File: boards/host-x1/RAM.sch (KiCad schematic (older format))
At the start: 0 parts

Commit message: Continued work on power supply
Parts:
- added U2: XC7A100T-1FTG256C, symbol XC7AxT-xFTG256x
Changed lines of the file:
@@
 $Descr A4 11693 8268
 encoding utf-8
-Sheet 1 4
+Sheet 3 5
 Title "STARSHIPRAIDER Single-Lane Host"
 Date "2017-05-04"
@@
 Comment4 ""
 $EndDescr
+$Comp
+L XC7AxT-xFTG256x U2
+U 6 1 590BFFBD
+P 1750 6050
+F 0 "U2" H 3128 8558 60  0000 L CNN
+F 1 "XC7A100T-1FTG256C" H 3128 8452 60  0000 L CNN
+F 2 "" H 1750 6050 60  0000 C CNN
+F 3 "" H 1750 6050 60  0000 C CNN
+	6    1750 6050
+	1    0    0    -1
+$EndComp
+$Comp
+L XC7AxT-xFTG256x U2
+U 5 1 590C013F
+P 4850 6000
+F 0 "U2" H 6228 8508 60  0000 L CNN
+F 1 "XC7A100T-1FTG256C" H 6228 8402 60  0000 L CNN
+F 2 "" H 4850 6000 60  0000 C CNN
+F 3 "" H 4850 6000 60  0000 C CNN
+	5    4850 6000
+	1    0    0    -1
+$EndComp
 $EndSCHEMATC

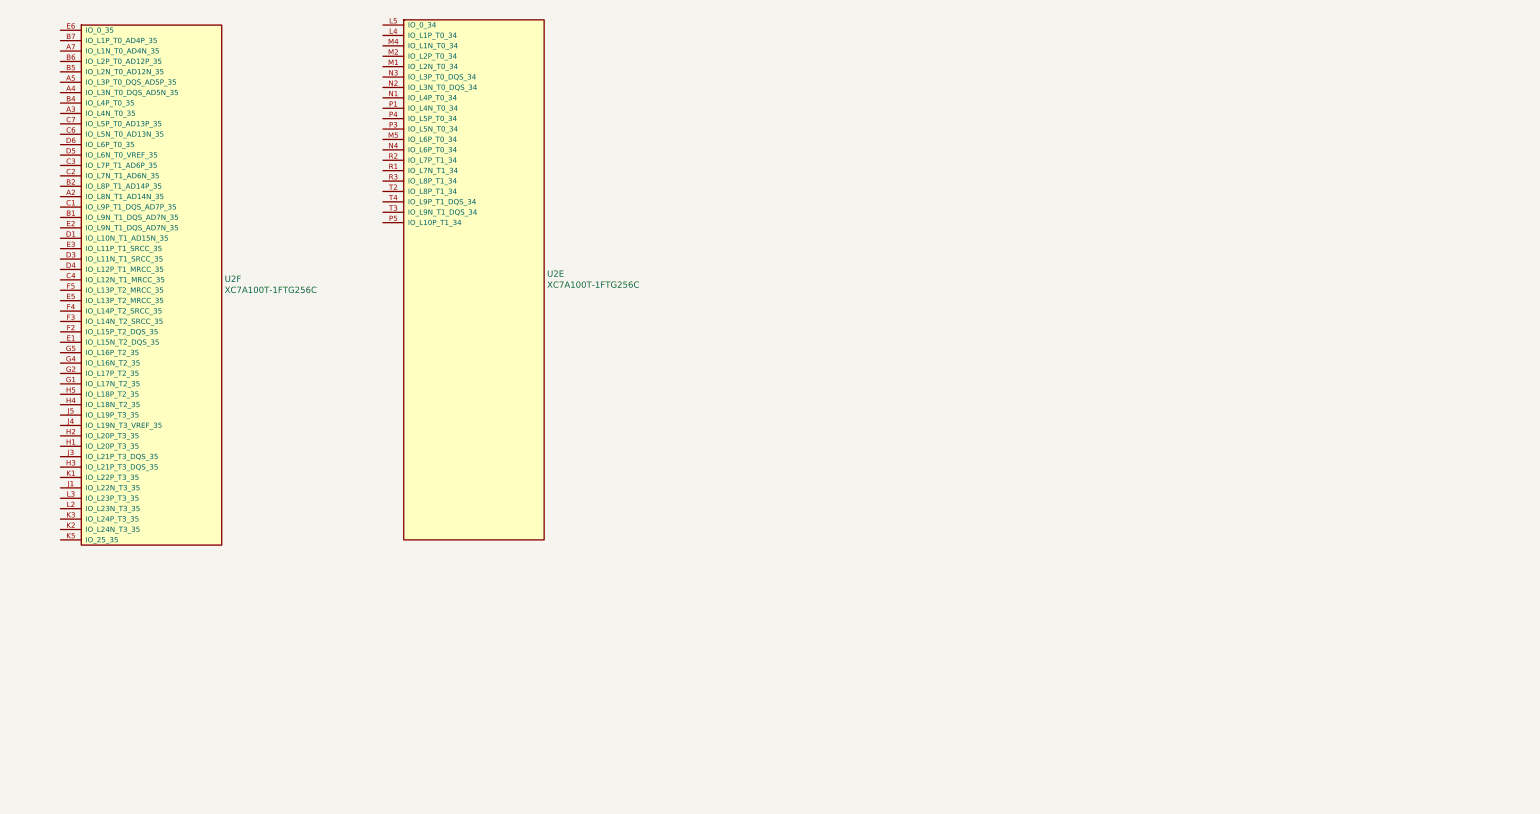
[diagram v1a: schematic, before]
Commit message: Initial work on RAM
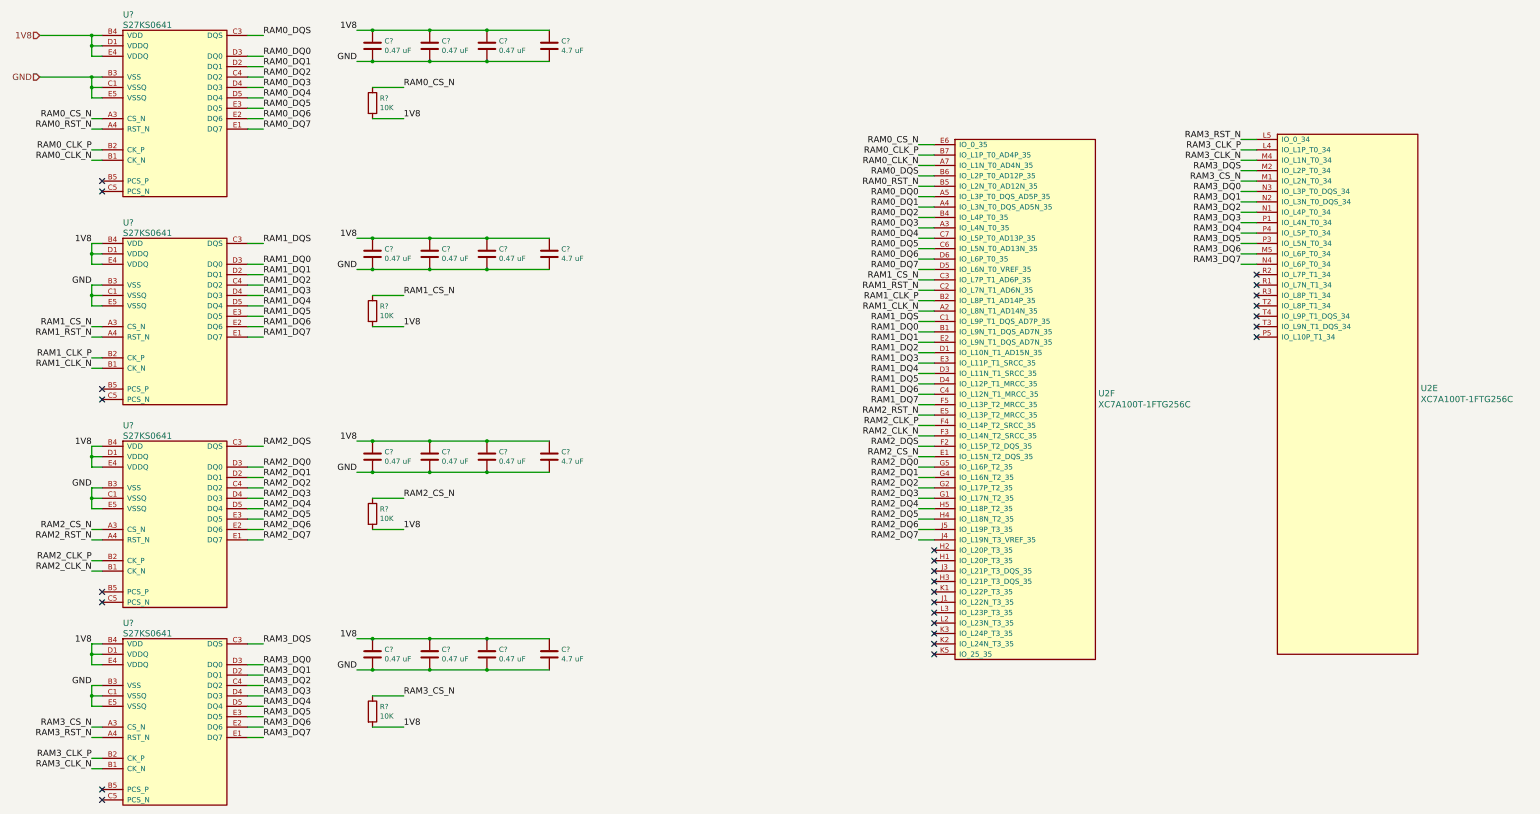
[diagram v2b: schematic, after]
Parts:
- added C? (x12): 0.47 uF, symbol C
- added C? (x4): 4.7 uF, symbol C
- added R? (x4): 10K, symbol R
- added U? (x4): S27KS0641, symbol S27KS0641
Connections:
- net RAM1_CLK_N: now reaches U2.A2 (IO_L8N_T1_AD14N_35)
- net RAM1_CLK_N: now also U?.B1 (CK_N)
- net RAM0_DQ3: now reaches U2.A3 (IO_L4N_T0_35)
- net RAM0_DQ3: now also U?.D4 (DQ3)
- net RAM0_DQ1: now reaches U2.A4 (IO_L3N_T0_DQS_AD5N_35)
- net RAM0_DQ1: now also U?.D2 (DQ1)
- net RAM0_DQ0: now reaches U2.A5 (IO_L3P_T0_DQS_AD5P_35)
- net RAM0_DQ0: now also U?.D3 (DQ0)
- net RAM0_CLK_N: now reaches U2.A7 (IO_L1N_T0_AD4N_35)
- net RAM0_CLK_N: now also U?.B1 (CK_N)
- net RAM1_DQ0: now reaches U2.B1 (IO_L9N_T1_DQS_AD7N_35)
- net RAM1_DQ0: now also U?.D3 (DQ0)
- net RAM1_CLK_P: now reaches U2.B2 (IO_L8P_T1_AD14P_35)
- net RAM1_CLK_P: now also U?.B2 (CK_P)
- net RAM0_DQ2: now reaches U2.B4 (IO_L4P_T0_35)
- net RAM0_DQ2: now also U?.C4 (DQ2)
- net RAM0_RST_N: now reaches U2.B5 (IO_L2N_T0_AD12N_35)
- net RAM0_RST_N: now also U?.A4 (RST_N)
- net RAM0_DQS: now reaches U2.B6 (IO_L2P_T0_AD12P_35)
- net RAM0_DQS: now also U?.C3 (DQS)
- net RAM0_CLK_P: now reaches U2.B7 (IO_L1P_T0_AD4P_35)
- net RAM0_CLK_P: now also U?.B2 (CK_P)
- net RAM1_DQS: now reaches U2.C1 (IO_L9P_T1_DQS_AD7P_35)
- net RAM1_DQS: now also U?.C3 (DQS)
- net RAM1_RST_N: now reaches U2.C2 (IO_L7N_T1_AD6N_35)
- net RAM1_RST_N: now also U?.A4 (RST_N)
- net RAM1_CS_N: now reaches U2.C3 (IO_L7P_T1_AD6P_35)
- net RAM1_CS_N: now also R?.1, U?.A3 (CS_N)
- net RAM1_DQ6: now reaches U2.C4 (IO_L12N_T1_MRCC_35)
- net RAM1_DQ6: now also U?.E2 (DQ6)
- net RAM0_DQ5: now reaches U2.C6 (IO_L5N_T0_AD13N_35)
- net RAM0_DQ5: now also U?.E3 (DQ5)
- net RAM0_DQ4: now reaches U2.C7 (IO_L5P_T0_AD13P_35)
- net RAM0_DQ4: now also U?.D5 (DQ4)
- net RAM1_DQ2: now reaches U2.D1 (IO_L10N_T1_AD15N_35)
- net RAM1_DQ2: now also U?.C4 (DQ2)
- net RAM1_DQ4: now reaches U2.D3 (IO_L11N_T1_SRCC_35)
- net RAM1_DQ4: now also U?.D5 (DQ4)
- net RAM1_DQ5: now reaches U2.D4 (IO_L12P_T1_MRCC_35)
- net RAM1_DQ5: now also U?.E3 (DQ5)
- net RAM0_DQ7: now reaches U2.D5 (IO_L6N_T0_VREF_35)
- net RAM0_DQ7: now also U?.E1 (DQ7)
- net RAM0_DQ6: now reaches U2.D6 (IO_L6P_T0_35)
- net RAM0_DQ6: now also U?.E2 (DQ6)
- net RAM2_CS_N: now reaches U2.E1 (IO_L15N_T2_DQS_35)
- net RAM2_CS_N: now also R?.1, U?.A3 (CS_N)
- net RAM1_DQ1: now reaches U2.E2 (IO_L9N_T1_DQS_AD7N_35)
- net RAM1_DQ1: now also U?.D2 (DQ1)
- net RAM1_DQ3: now reaches U2.E3 (IO_L11P_T1_SRCC_35)
- net RAM1_DQ3: now also U?.D4 (DQ3)
- net RAM2_RST_N: now reaches U2.E5 (IO_L13P_T2_MRCC_35)
- net RAM2_RST_N: now also U?.A4 (RST_N)
- net RAM0_CS_N: now reaches U2.E6 (IO_0_35)
- net RAM0_CS_N: now also R?.1, U?.A3 (CS_N)
- net RAM2_DQS: now reaches U2.F2 (IO_L15P_T2_DQS_35)
- net RAM2_DQS: now also U?.C3 (DQS)
- net RAM2_CLK_N: now reaches U2.F3 (IO_L14N_T2_SRCC_35)
- net RAM2_CLK_N: now also U?.B1 (CK_N)
- net RAM2_CLK_P: now reaches U2.F4 (IO_L14P_T2_SRCC_35)
- net RAM2_CLK_P: now also U?.B2 (CK_P)
- net RAM1_DQ7: now reaches U2.F5 (IO_L13P_T2_MRCC_35)
- net RAM1_DQ7: now also U?.E1 (DQ7)
- net RAM2_DQ3: now reaches U2.G1 (IO_L17N_T2_35)
- net RAM2_DQ3: now also U?.D4 (DQ3)
- net RAM2_DQ2: now reaches U2.G2 (IO_L17P_T2_35)
- net RAM2_DQ2: now also U?.C4 (DQ2)
- net RAM2_DQ1: now reaches U2.G4 (IO_L16N_T2_35)
- net RAM2_DQ1: now also U?.D2 (DQ1)
- net RAM2_DQ0: now reaches U2.G5 (IO_L16P_T2_35)
- net RAM2_DQ0: now also U?.D3 (DQ0)
- net RAM2_DQ5: now reaches U2.H4 (IO_L18N_T2_35)
- net RAM2_DQ5: now also U?.E3 (DQ5)
- net RAM2_DQ4: now reaches U2.H5 (IO_L18P_T2_35)
- net RAM2_DQ4: now also U?.D5 (DQ4)
- net RAM2_DQ7: now reaches U2.J4 (IO_L19N_T3_VREF_35)
- net RAM2_DQ7: now also U?.E1 (DQ7)
- net RAM2_DQ6: now reaches U2.J5 (IO_L19P_T3_35)
- net RAM2_DQ6: now also U?.E2 (DQ6)
- net RAM3_CLK_P: now reaches U2.L4 (IO_L1P_T0_34)
- net RAM3_CLK_P: now also U?.B2 (CK_P)
- net RAM3_RST_N: now reaches U2.L5 (IO_0_34)
- net RAM3_RST_N: now also U?.A4 (RST_N)
- net RAM3_CS_N: now reaches U2.M1 (IO_L2N_T0_34)
- net RAM3_CS_N: now also R?.1, U?.A3 (CS_N)
- net RAM3_DQS: now reaches U2.M2 (IO_L2P_T0_34)
- net RAM3_DQS: now also U?.C3 (DQS)
- net RAM3_CLK_N: now reaches U2.M4 (IO_L1N_T0_34)
- net RAM3_CLK_N: now also U?.B1 (CK_N)
- net RAM3_DQ6: now reaches U2.M5 (IO_L6P_T0_34)
- net RAM3_DQ6: now also U?.E2 (DQ6)
- net RAM3_DQ2: now reaches U2.N1 (IO_L4P_T0_34)
- net RAM3_DQ2: now also U?.C4 (DQ2)
- net RAM3_DQ1: now reaches U2.N2 (IO_L3N_T0_DQS_34)
- net RAM3_DQ1: now also U?.D2 (DQ1)
- net RAM3_DQ0: now reaches U2.N3 (IO_L3P_T0_DQS_34)
- net RAM3_DQ0: now also U?.D3 (DQ0)
- net RAM3_DQ7: now reaches U2.N4 (IO_L6P_T0_34)
- net RAM3_DQ7: now also U?.E1 (DQ7)
- net RAM3_DQ3: now reaches U2.P1 (IO_L4N_T0_34)
- net RAM3_DQ3: now also U?.D4 (DQ3)
- net RAM3_DQ5: now reaches U2.P3 (IO_L5N_T0_34)
- net RAM3_DQ5: now also U?.E3 (DQ5)
- net RAM3_DQ4: now reaches U2.P4 (IO_L5P_T0_34)
- net RAM3_DQ4: now also U?.D5 (DQ4)
- new net 1V8: C?.1, C?.1, C?.1, C?.1, C?.1, C?.1, C?.1, C?.1, C?.1, C?.1, C?.1, C?.1, C?.1, C?.1, C?.1, C?.1, R?.2, R?.2, R?.2, R?.2, U?.B4 (VDD), U?.B4 (VDD), U?.B4 (VDD), U?.B4 (VDD), U?.D1 (VDDQ), U?.D1 (VDDQ), U?.D1 (VDDQ), U?.D1 (VDDQ), U?.E4 (VDDQ), U?.E4 (VDDQ), U?.E4 (VDDQ), U?.E4 (VDDQ)
- new net GND: C?.2, C?.2, C?.2, C?.2, C?.2, C?.2, C?.2, C?.2, C?.2, C?.2, C?.2, C?.2, C?.2, C?.2, C?.2, C?.2, U?.B3 (VSS), U?.B3 (VSS), U?.B3 (VSS), U?.B3 (VSS), U?.C1 (VSSQ), U?.C1 (VSSQ), U?.C1 (VSSQ), U?.C1 (VSSQ), U?.E5 (VSSQ), U?.E5 (VSSQ), U?.E5 (VSSQ), U?.E5 (VSSQ)
- no-connect marks 0 -> 26
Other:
- moved on the sheet: U2E, U2F
